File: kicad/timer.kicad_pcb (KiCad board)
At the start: 2 copper layers, 70 x 100 mm, 27 parts, among them IC1 ATMEGA328P-A, P1 BATTERY, P2 ICSP, Q1 NMOS, Q2 PMOS, SW1 SPST, U1 TOUCH_PAD_13, U2 MTCH6102_SSOP, U3 MCP1755ST-3302E/DB, U4 APA_102C

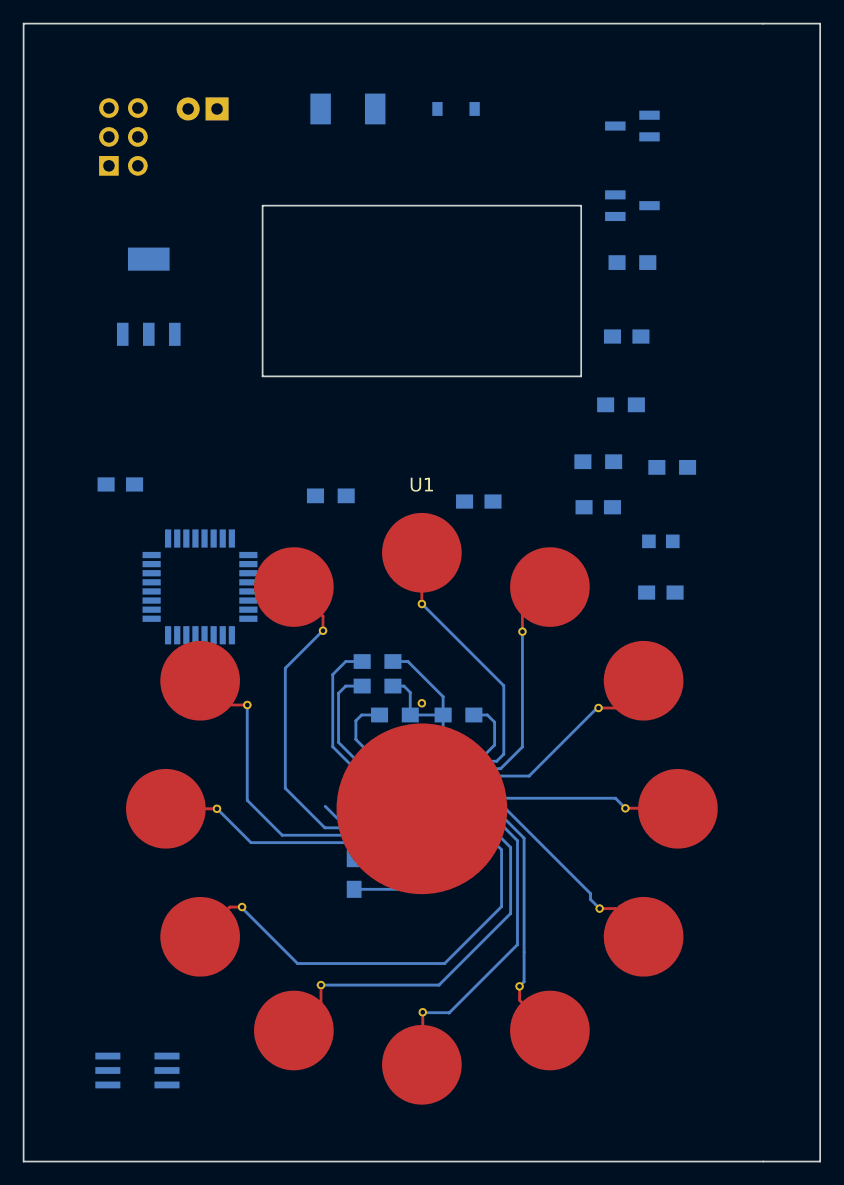
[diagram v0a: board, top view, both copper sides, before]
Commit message: More squeezing
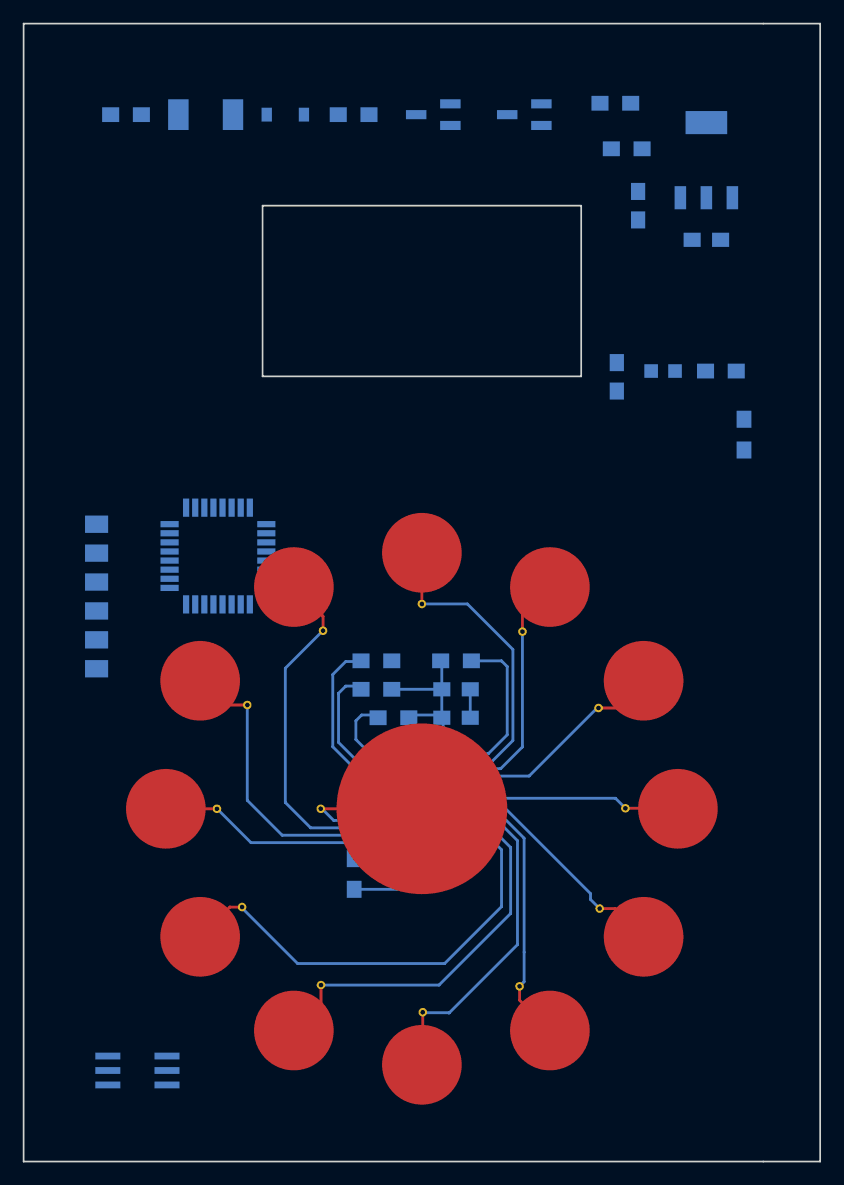
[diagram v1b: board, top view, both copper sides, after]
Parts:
- P1: footprint Pin_Headers:Pin_Header_Straight_1x02 -> Resistors_SMD:R_0805_HandSoldering
- P2: footprint Pin_Headers:Pin_Header_Straight_2x03 -> SIP-6-SMD
- U1: footprint touch_timer:touch_circle -> touch_circle
- moved U3 50.4 mm to (175.0, 47.0)
- moved R6 40.1 mm to (168.0, 46.0)
- moved P2 37.9 mm to (121.4, 85.3), turned to 90 degrees
- moved C2 34.6 mm to (153.0, 93.5)
- moved R7 31.5 mm to (167.0, 42.0)
- moved C4 29.5 mm to (169.0, 51.0), turned to 270 degrees
- moved R8 27.7 mm to (144.0, 43.0)
- moved C1 22.3 mm to (153.0, 96.0)
- moved C5 19.4 mm to (167.1, 66.0), turned to 90 degrees
- moved Q2 19.2 mm to (151.0, 43.0), turned to 270 degrees
- moved D1 15.0 mm to (138.0, 43.0), turned to 180 degrees
- moved D2 15.0 mm to (171.2, 65.5)
- moved SW1 12.5 mm to (131.0, 43.0), turned to 180 degrees
- moved R10 11.1 mm to (178.3, 71.1), turned to 90 degrees
- moved C3 11.0 mm to (175.0, 54.0), turned to 180 degrees
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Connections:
- R4 pad 1: Net-(R4-Pad1) -> /3V3
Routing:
- net /RX12: track 6.01 -> 15.0 mm
- net /SCL: track 6.61 -> 13.4 mm
- net /RX0: track 24.0 -> 26.8 mm
- net GND: track 0.00 -> 2.50 mm
- net Net-(R4-Pad1): track 1.32 -> 0.00 mm
- net /RX11: track 30.6 -> 31.3 mm
